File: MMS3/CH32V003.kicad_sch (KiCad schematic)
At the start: 9 parts, among them J3 Program, U8 CH32V003FxPx, X1 X322525MOB4SI

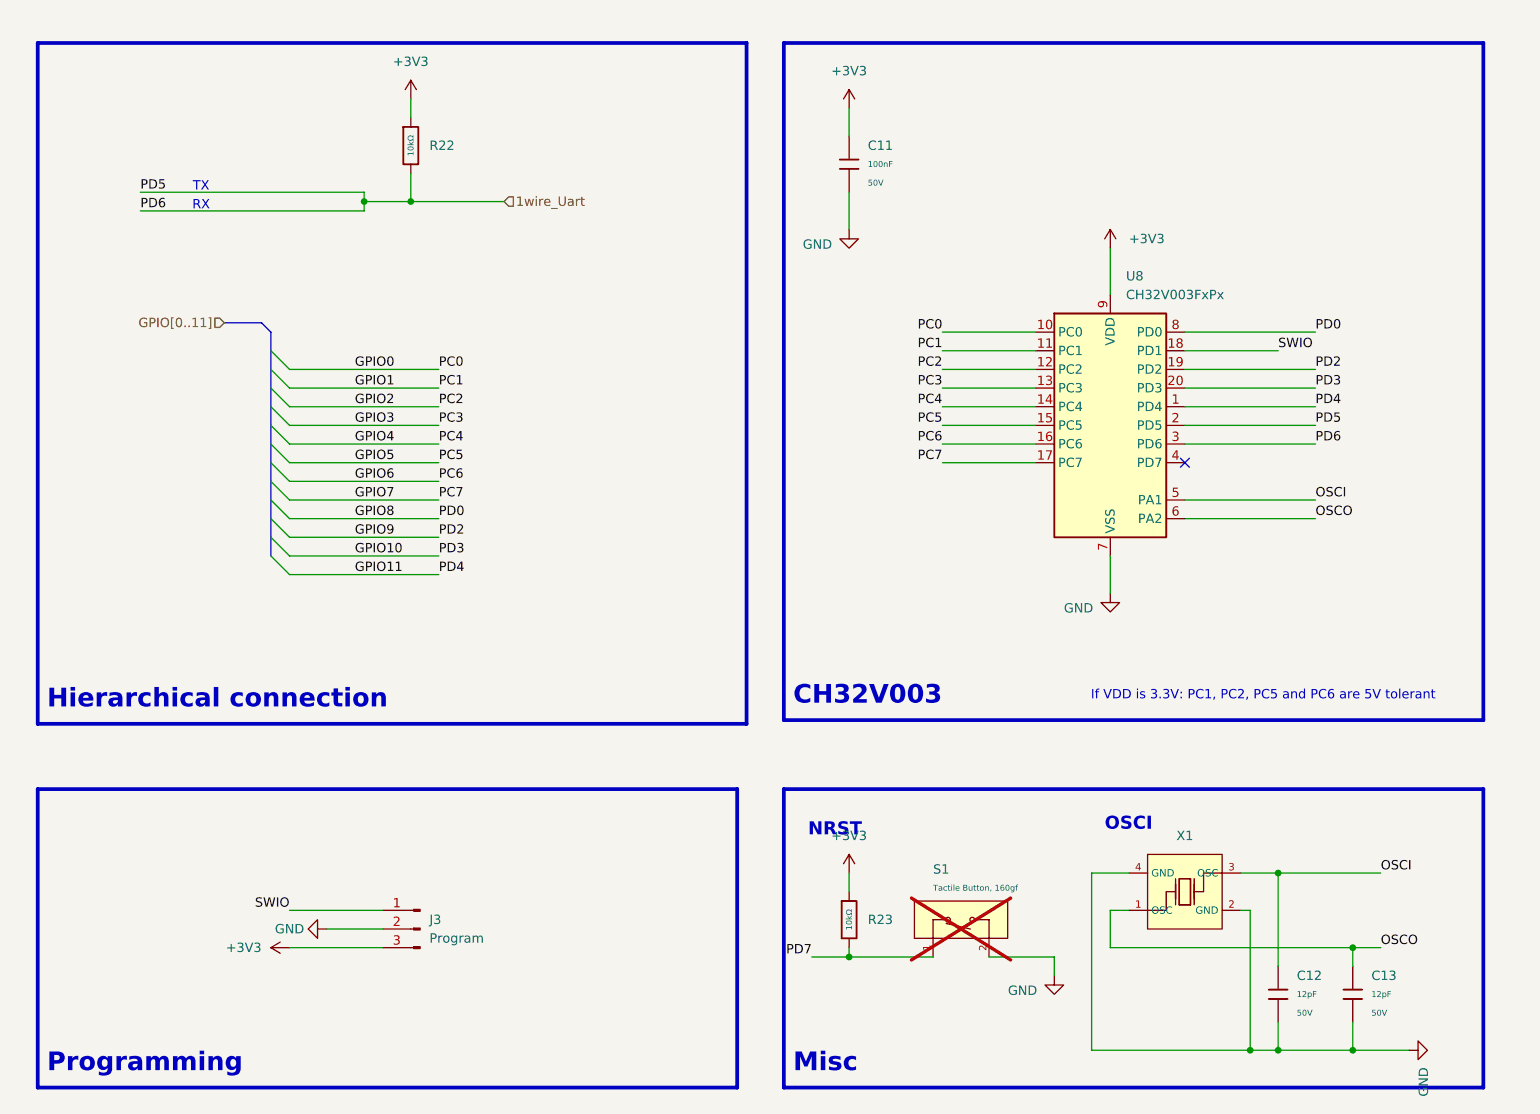
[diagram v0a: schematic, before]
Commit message: backup commit
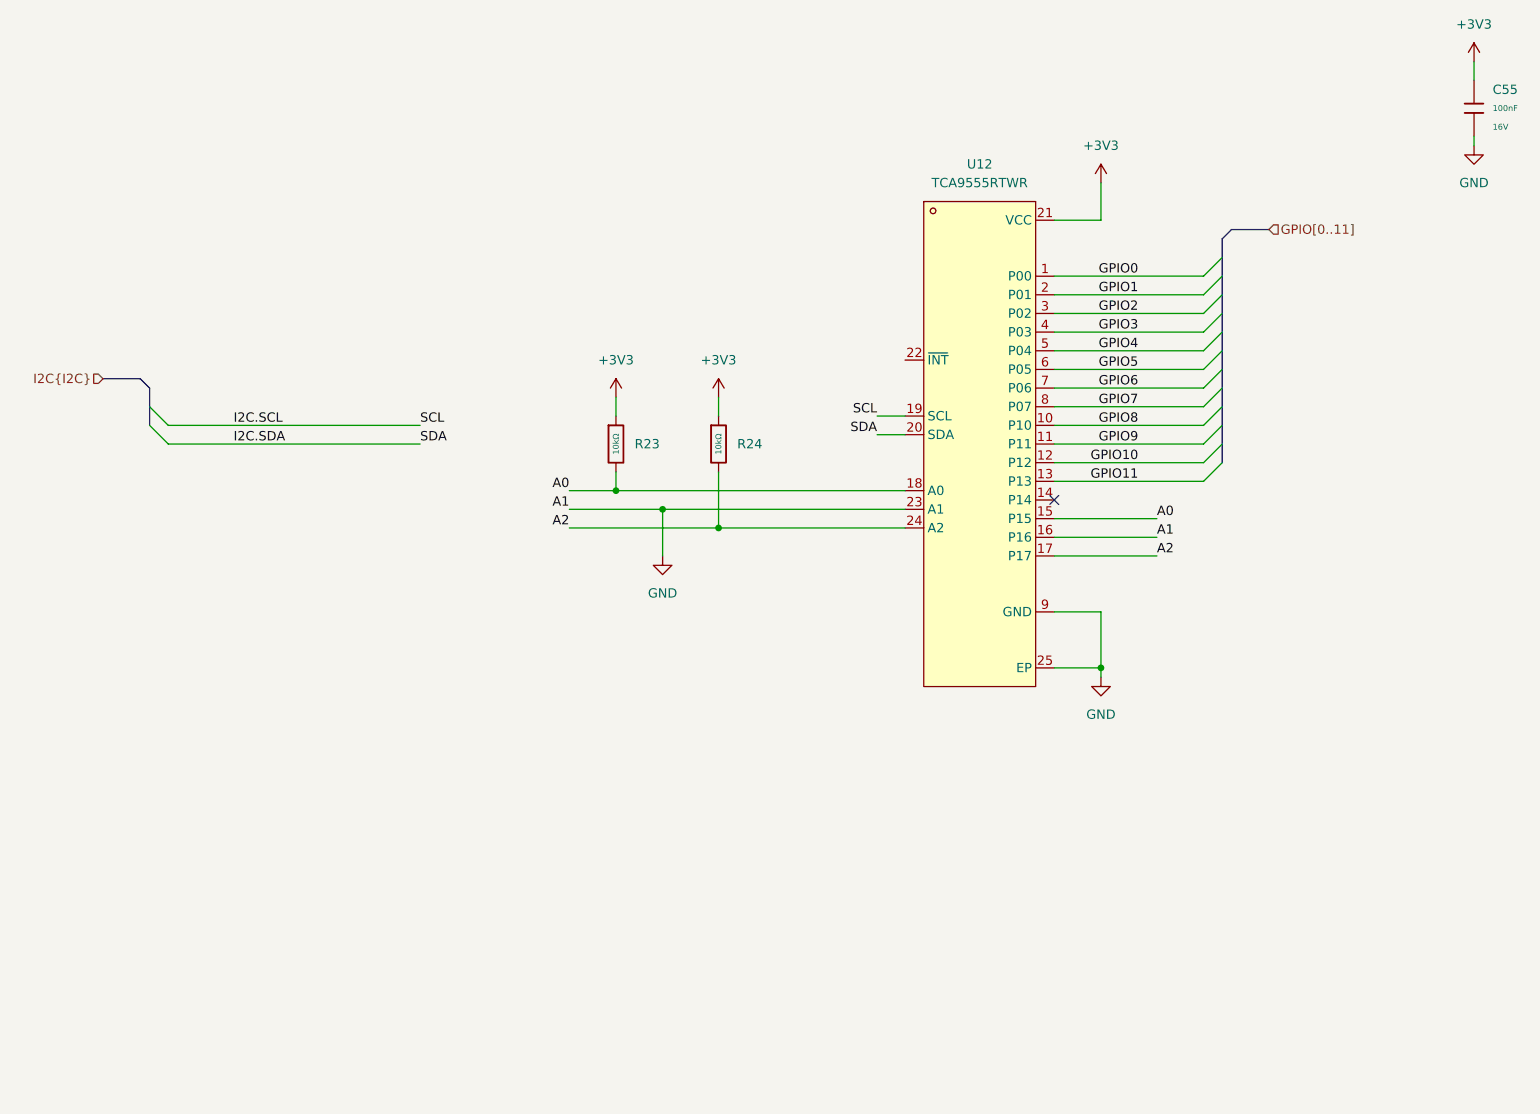
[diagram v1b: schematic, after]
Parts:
- removed C11: 100nF, PCM_JLCPCB:C_0603, symbol PCM_JLCPCB-Capacitors:0603,100nF
- removed C12, C13: 12pF, PCM_JLCPCB:C_0603, symbol PCM_JLCPCB-Capacitors:0603,12pF
- removed J3: Program, Connector_PinHeader_2.54mm:PinHeader_1x03_P2.54mm_Vertical, symbol Connector:Conn_01x03_Pin
- removed R22, R23: 10kΩ, PCM_JLCPCB:R_0603, symbol PCM_JLCPCB-Resistors:0603,10kΩ
- removed S1: Tactile Button, 160gf, PCM_JLCPCB:SW_TS-1088-AR02016, symbol PCM_JLCPCB-Connectors_Buttons:Tactile Button, 160gf, 12V, 50mA, 4.0mm
- removed U8: CH32V003FxPx, PCM_JLCPCB:TSSOP-20_4.4x6.5mm_P0.65mm, symbol MCU_WCH_RiscV:CH32V003FxPx
- removed X1: X322525MOB4SI, PCM_JLCPCB:OSC-SMD_4P-L3.2-W2.5-BL, symbol PCM_JLCPCB-Crystals:Crystal, 25MHz, 11pF
- added C55: 100nF, PCM_JLCPCB:C_0402, symbol PCM_JLCPCB-Capacitors:0402,100nF
- added R23, R24: 10kΩ, PCM_JLCPCB:R_0402, symbol PCM_JLCPCB-Resistors:0402,10kΩ
- added U12: TCA9555RTWR, I2C_GPIO:HVQFN-24_L4.0-W4.0-P0.50-BL-EP2.6, symbol I2C_GPIO:TCA9555RTWR
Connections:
- net +3V3: now also C55.1, R23.1, R24.1, U12.21 (VCC)
- net GND: now also C55.2, U12.16 (P16), U12.23 (A1), U12.25 (EP), U12.9 (GND)
- net GPIO0: now also U12.1 (P00)
- net GPIO1: now also U12.2 (P01)
- net GPIO10: now also U12.12 (P12)
- net GPIO11: now also U12.13 (P13)
- net GPIO2: now also U12.3 (P02)
- net GPIO3: now also U12.4 (P03)
- net GPIO4: now also U12.5 (P04)
- net GPIO5: now also U12.6 (P05)
- net GPIO6: now also U12.7 (P06)
- net GPIO7: now also U12.8 (P07)
- net GPIO8: now also U12.10 (P10)
- net GPIO9: now also U12.11 (P11)
- new net A0: R23.2, U12.15 (P15), U12.18 (A0)
- new net A2: R24.2, U12.17 (P17), U12.24 (A2)
- new net I2C.SCL: U12.19 (SCL)
- new net I2C.SDA: U12.20 (SDA)
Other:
- note removed: "CH32V003"
- note removed: "Hierarchical connection"
- note removed: "If VDD is 3.3V: PC1, PC2, PC5 and PC6 are 5V tolerant"
- note removed: "Misc"
- note removed: "NRST"
- note removed: "OSCI"
- note removed: "Programming"
- note removed: "RX"
- note removed: "TX"
